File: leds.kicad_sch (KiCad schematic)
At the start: 24 parts, among them IC1 SN74LV1T34DCKR

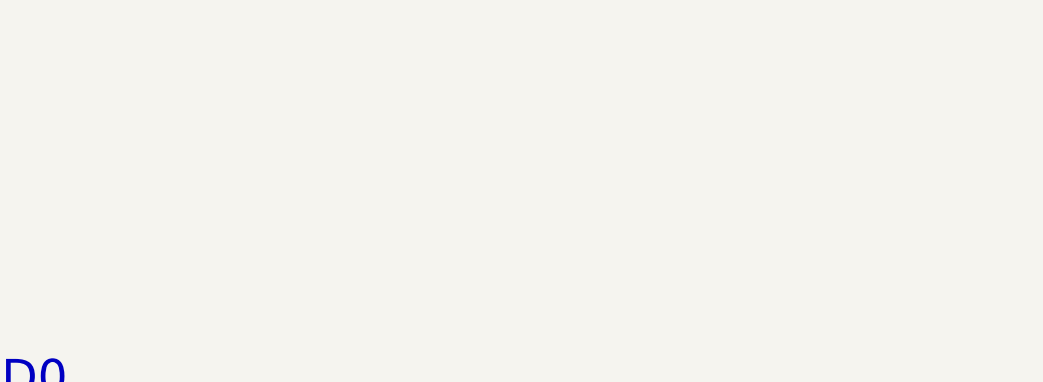
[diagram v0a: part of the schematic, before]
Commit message: 2.1
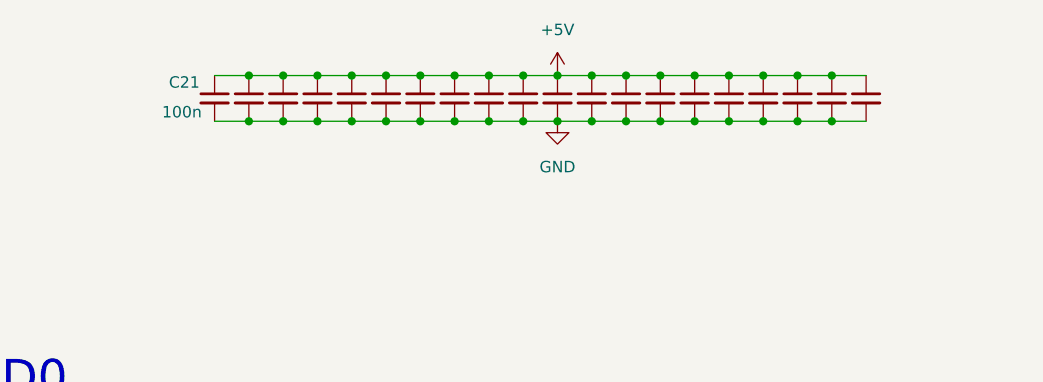
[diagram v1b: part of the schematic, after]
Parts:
- added C21, C29, C30, C31, C32, C33, C34, C35, C36, C37, C38, C39, C40, C41, C42, C43, C44, C45, C46, C47: 100n, Capacitor_SMD:C_0603_1608Metric, symbol Device:C_Small
- D10, D11, D12, D13, D14, D15, D16, D17, D18, D19, D20, D21, D22, D3, D4, D5, D6, D7, D8, D9: footprint LED_SMD:LED_WS2812B_PLCC4_5.0x5.0mm_P3.2mm -> Library_local:LED_WS2812B-2020_PLCC4_2.0x2.0mm
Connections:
- net +5V: now also C21.1, C29.1, C30.1, C31.1, C32.1, C33.1, C34.1, C35.1, C36.1, C37.1, C38.1, C39.1, C40.1, C41.1, C42.1, C43.1, C44.1, C45.1, C46.1, C47.1
- net GND: now also C21.2, C29.2, C30.2, C31.2, C32.2, C33.2, C34.2, C35.2, C36.2, C37.2, C38.2, C39.2, C40.2, C41.2, C42.2, C43.2, C44.2, C45.2, C46.2, C47.2
